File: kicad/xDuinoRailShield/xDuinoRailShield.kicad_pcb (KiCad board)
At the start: 2 copper layers, 43.2 x 18.9 mm, 31 parts, among them J106 21mtc_mrkl, Q401 S8050, Q402 S8550, Q403 S8550, Q404 S8050, U501 MOUDLE-SEEEDUINO-XIAO-ESP32C3, U701 L78L05_SOT89, U801 BDR6133, U803 ULN2003A, U902 LIS3DH

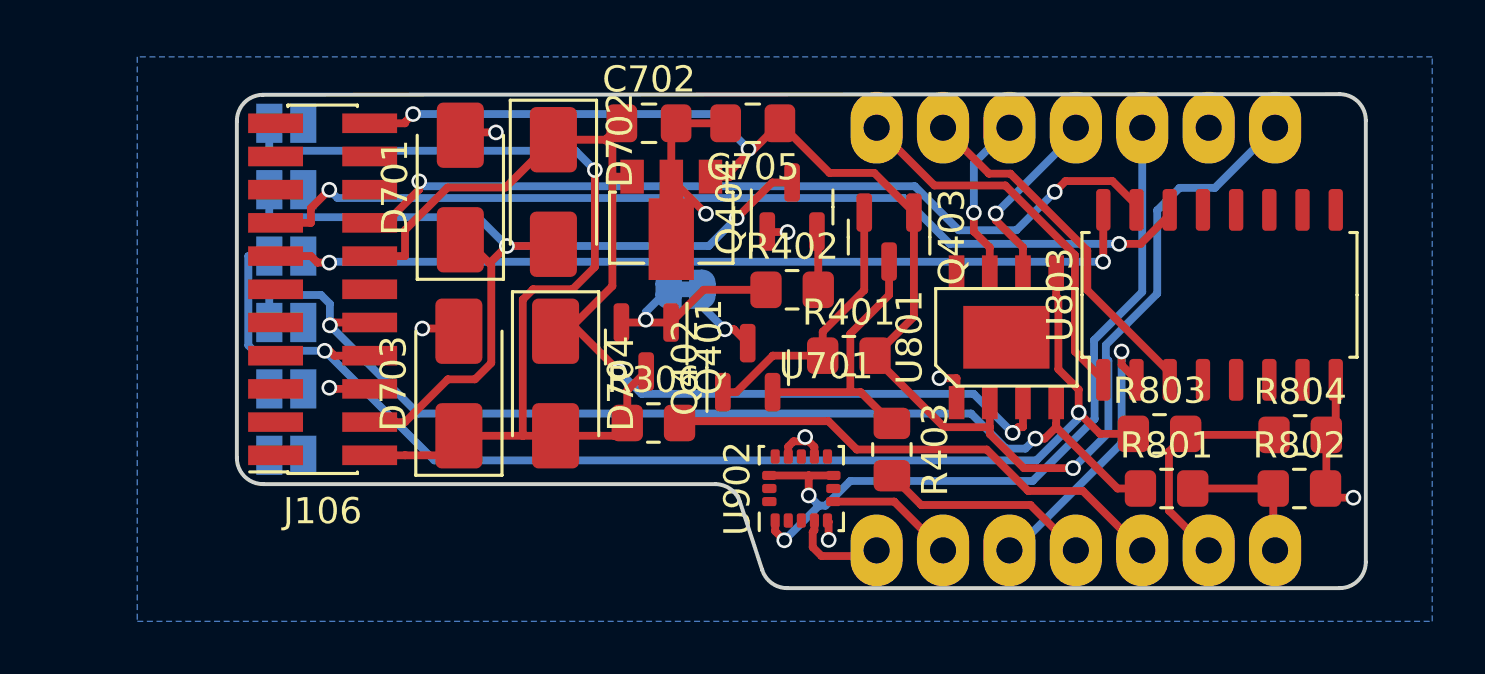
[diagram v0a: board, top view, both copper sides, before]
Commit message: Refactoring & Sound
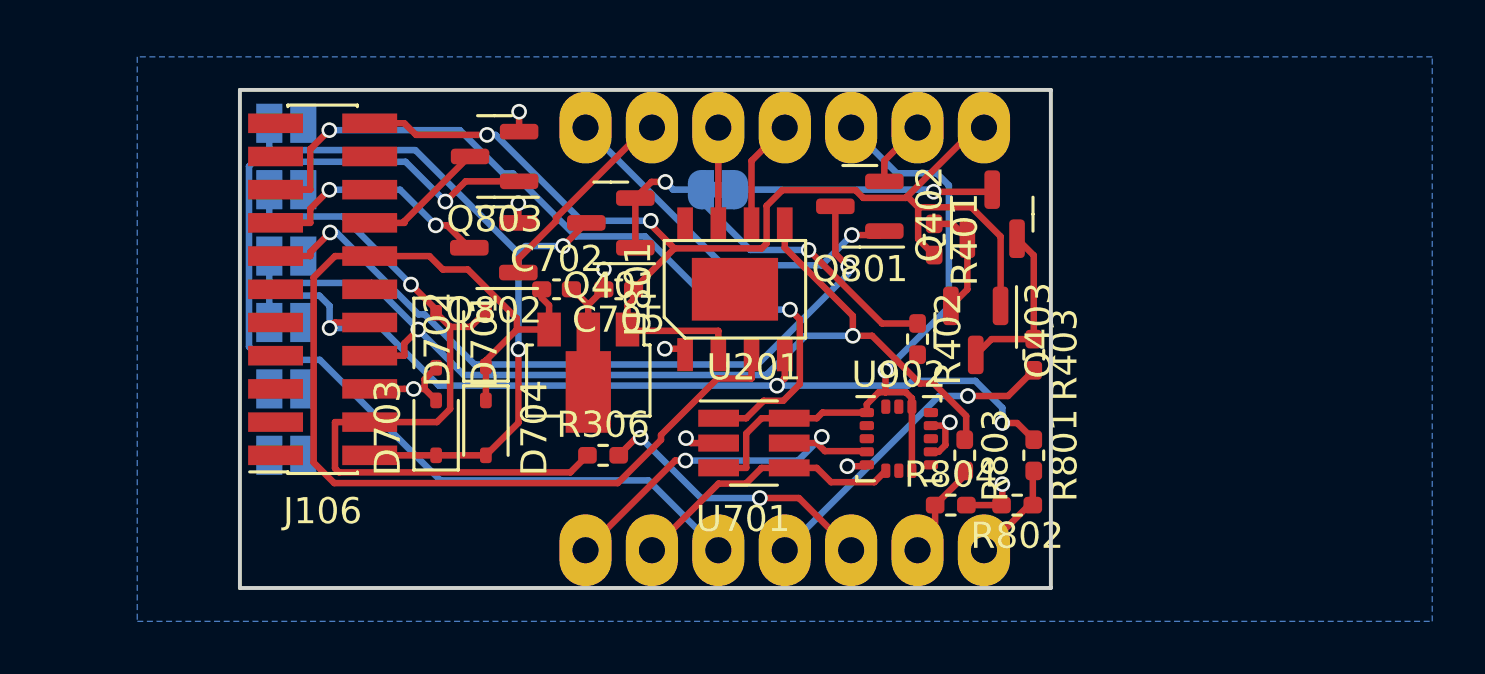
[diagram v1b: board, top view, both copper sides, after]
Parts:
- removed Q404: S8050, Package_TO_SOT_SMD:SOT-23
- removed U803: ULN2003A, Package_SO:SOIC-16_4.55x10.3mm_P1.27mm
- added Q801: 2N7002, Package_TO_SOT_SMD:SOT-23, F.Cu at (148.0, 71.4)
- added Q802: 2N7002, Package_TO_SOT_SMD:SOT-23, F.Cu at (134.0, 73.0)
- added Q803: 2N7002, Package_TO_SOT_SMD:SOT-23, F.Cu at (134.0, 69.5)
- added U201: MCP4725xxx-xCH, Package_TO_SOT_SMD:SOT-23-6_Handsoldering, F.Cu at (143.9, 80.5)
- C702, C705: footprint Capacitor_SMD:C_0805_2012Metric_Pad1.18x1.45mm_HandSolder -> Capacitor_SMD:C_0402_1005Metric_Pad0.74x0.62mm_HandSolder
- D701, D702, D703, D704: value SS34 -> 1N5819WS; footprint Diode_SMD:D_SMA -> Diode_SMD:D_SOD-323
- R306, R401, R402, R403, R801, R802, R803, R804: footprint Resistor_SMD:R_0805_2012Metric_Pad1.20x1.40mm_HandSolder -> Resistor_SMD:R_0402_1005Metric_Pad0.72x0.64mm_HandSolder
- moved R804 13.6 mm to (151.4, 82.9)
- moved U501 11.1 mm to (134.6, 85.4)
- moved Q402 11.0 mm to (153.0, 71.7)
- moved R802 10.8 mm to (154.0, 82.9), turned to 180 degrees
- moved U801 10.5 mm to (143.2, 74.6)
- moved C705 8.16 mm to (138.7, 74.6)
- moved R803 7.50 mm to (152.0, 81.0), turned to -90 degrees
- moved C702 7.27 mm to (136.4, 74.6)
- moved U701 6.65 mm to (137.6, 78.1)
- moved R403 6.53 mm to (154.6, 77.1)
- moved D702 6.19 mm to (133.7, 76.5), turned to 90 degrees
- moved D701 5.92 mm to (131.8, 76.5), turned to -90 degrees
- moved R401 5.51 mm to (150.8, 72.7), turned to -90 degrees
- moved R801 5.24 mm to (154.6, 81.0), turned to -90 degrees
- moved R402 5.15 mm to (150.2, 76.5), turned to -90 degrees
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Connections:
- net /Connectors 21mtc / PluXX / NEMA/SPEAKER1 renamed /Audio Interfaces/SPEAKER1
- net /MCU Carrier Board/I2C0 renamed /Audio Interfaces/I2C0
- net /MCU Carrier Board/I2C1 renamed /Audio Interfaces/I2C1
- net DCC_VIN renamed U+
- J106 pad 17: /Connectors 21mtc / PluXX / NEMA/SPEAKER0 -> /Audio Interfaces/SPEAKER0
- R306 pad 1: /DCC1 -> /DCC0
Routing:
- net /Audio Interfaces/SPEAKER0: track 0.00 -> 31.0 mm, vias 0 -> 2
- net /AUX1: track 10.8 -> 39.4 mm
- net /Connectors 21mtc / PluXX / NEMA/AMP_FUNC1: track 36.6 -> 9.17 mm
- net /Connectors 21mtc / PluXX / NEMA/AMP_AUX1: track 32.3 -> 4.93 mm, vias 2 -> 0
- net +5V: track 59.2 -> 45.8 mm, vias 3 -> 2
- net /DCC1: track 38.6 -> 28.0 mm, vias 1 -> 2
- net /Audio Interfaces/I2C0: track 3.72 -> 14.3 mm, vias 0 -> 2
- net DCC_MM: track 19.8 -> 11.0 mm, vias 0 -> 2
- net /Connectors 21mtc / PluXX / NEMA/AMP_MOTOR1: track 48.6 -> 39.9 mm
- net /Railcom-Feedback/RC_SIGNAL: track 7.66 -> 15.4 mm, vias 1 -> 2
- net Net-(JP401-A): track 2.98 -> 9.91 mm
- net /Railcom-Feedback/RC_CURR: track 10.5 -> 4.34 mm
- net /MCU Carrier Board/FUNC1: track 13.7 -> 7.79 mm
- net /Audio Interfaces/I2C1: track 4.97 -> 10.7 mm
- net /DCC0: track 36.2 -> 30.9 mm, vias 2 -> 1
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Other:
- board size 43.2 x 18.9 mm -> 31 x 19.1 mm

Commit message: More refactoring
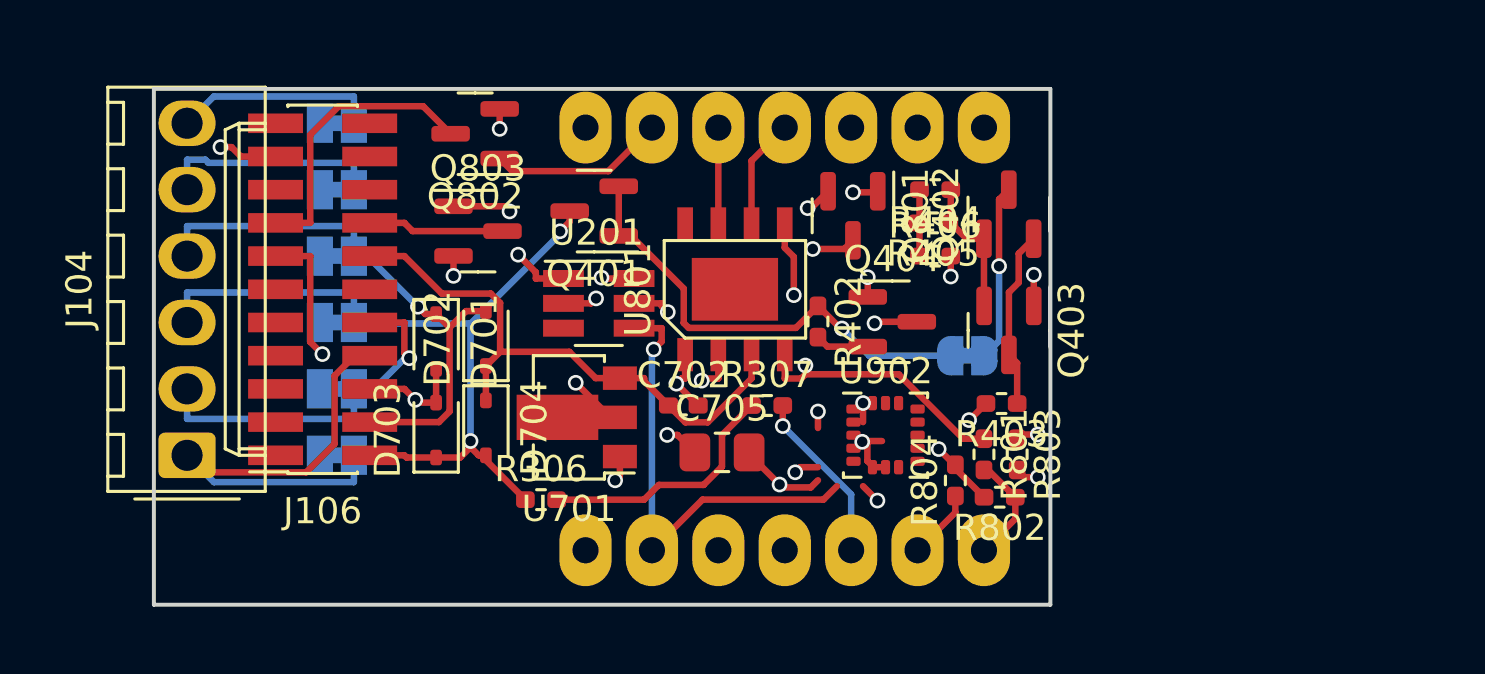
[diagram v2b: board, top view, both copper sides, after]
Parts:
- removed R401: 20, Resistor_SMD:R_0402_1005Metric_Pad0.72x0.64mm_HandSolder
- added J104: Conn_01x06, Connector_Molex:Molex_KK-254_AE-6410-06A_1x06_P2.54mm_Vertical, F.Cu at (122.2, 81.0)
- added Q404: S8050, Package_TO_SOT_SMD:SOT-23, F.Cu at (149.2, 75.8)
- added R307: 10k, Resistor_SMD:R_0402_1005Metric_Pad0.72x0.64mm_HandSolder, F.Cu at (144.4, 79.0)
- added R404: 10R, Resistor_SMD:R_0402_1005Metric_Pad0.72x0.64mm_HandSolder, F.Cu at (150.8, 70.8)
- added R405: 10R, Resistor_SMD:R_0402_1005Metric_Pad0.72x0.64mm_HandSolder, F.Cu at (150.8, 72.1)
- added R406: 10R, Resistor_SMD:R_0402_1005Metric_Pad0.72x0.64mm_HandSolder, F.Cu at (150.8, 73.3)
- C705: footprint Capacitor_SMD:C_0402_1005Metric_Pad0.74x0.62mm_HandSolder -> Capacitor_SMD:C_0805_2012Metric_Pad1.18x1.45mm_HandSolder
- R306: value 22k -> 10k
- R402: value 6k8 -> 10k
- R801, R803: value 6K8 -> 10k
- U701: value L78L05_SOT89 -> HT7533-1
- moved JP102 12.8 mm to (128.0, 81.0), turned to 0 degrees
- moved JP106 12.8 mm to (128.0, 68.2), turned to 0 degrees
- moved JP401 11.5 mm to (152.1, 77.1)
- moved U201 7.98 mm to (138.0, 75.1)
- moved JP101 7.86 mm to (128.0, 78.4), turned to 0 degrees
- moved JP105 7.86 mm to (128.0, 70.8), turned to 0 degrees
- moved C705 7.38 mm to (142.7, 80.8), turned to 0 degrees
- moved C702 6.58 mm to (141.2, 79.0)
- moved Q802 4.42 mm to (133.2, 68.7)
- moved R402 3.87 mm to (146.4, 75.8)
- moved JP103 3.19 mm to (128.0, 73.3), turned to 0 degrees
- moved JP104 3.19 mm to (128.0, 75.9), turned to 0 degrees
- moved Q803 2.92 mm to (133.4, 72.4), turned to 0 degrees
- moved R306 2.92 mm to (135.8, 82.6)
- moved R403 2.24 mm to (153.4, 79.0), turned to 180 degrees
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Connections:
- C705 pad 1: +5V -> +3V3
- J106 pad 22: +5V -> /Connectors 21mtc / PluXX / NEMA/+3V3
- JP101 pad 2: /DCC0 -> /Connectors 21mtc / PluXX / NEMA/AMP_MOTOR0
- JP102 pad 2: /DCC1 -> /Connectors 21mtc / PluXX / NEMA/AMP_MOTOR1
- JP103 pad 2: /Connectors 21mtc / PluXX / NEMA/AMP_MOTOR0 -> /DCC0
- JP104 pad 2: /Connectors 21mtc / PluXX / NEMA/AMP_MOTOR1 -> /DCC1
- JP105 pad 2: /Connectors 21mtc / PluXX / NEMA/FUNC0 -> /Connectors 21mtc / PluXX / NEMA/FUNC1
- JP106 pad 2: /Connectors 21mtc / PluXX / NEMA/FUNC1 -> /Connectors 21mtc / PluXX / NEMA/FUNC0
- Q403 pad 1: +5V -> +3V3
- R306 pad 1: /DCC0 -> /DCC1
- R306 pad 2: DCC_MM -> Net-(R306-Pad2)
- U201 pad 1: /Audio Interfaces/SPEAKER0 -> /Audio Interfaces/SPEAKER1
- U701 pad 1: +5V -> +3V3
- U801 pad 2: +5V -> +3V3
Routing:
- net +5V: track 45.8 -> 0.00 mm, vias 2 -> 0
- net /Audio Interfaces/SPEAKER0: track 31.0 -> 0.00 mm, vias 2 -> 0
- net /AUX1: track 39.4 -> 18.7 mm
- net U+: track 42.4 -> 22.1 mm
- net /Connectors 21mtc / PluXX / NEMA/AMP_MOTOR1: track 39.9 -> 59.6 mm
- net /Audio Interfaces/SPEAKER1: track 0.00 -> 17.6 mm, vias 0 -> 2
- net +3V3: track 26.0 -> 9.27 mm, vias 1 -> 9
- net /DCC0: track 30.9 -> 42.1 mm, vias 1 -> 2
- net Net-(R306-Pad2): track 0.00 -> 9.65 mm
- net /Connectors 21mtc / PluXX / NEMA/FUNC1: track 0.00 -> 8.60 mm
- net /Connectors 21mtc / PluXX / NEMA/FUNC0: track 0.00 -> 7.83 mm
- net /Audio Interfaces/I2C1: track 10.7 -> 17.8 mm, vias 0 -> 1
- net /Audio Interfaces/I2C0: track 14.3 -> 19.9 mm
- net /MCU Carrier Board/EMF_MOTOR1: track 3.78 -> 9.34 mm, vias 0 -> 1
- net DCC_MM: track 11.0 -> 6.62 mm, vias 2 -> 1
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- added copper zone on In2.Cu, net +3V3
- added copper zone on In1.Cu, net GND
- removed copper zone on B.Cu, net GND
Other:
- board size 31 x 19.1 mm -> 34.3 x 19.7 mm
- copper layers 2 -> 4
